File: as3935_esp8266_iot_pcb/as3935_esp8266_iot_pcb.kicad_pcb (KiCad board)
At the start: 2 copper layers, 50 x 100 mm, 44 parts, among them K1 RELAY_2RT, K2 RELAY_2RT, P1 CONN_01X02, P10 CONN_01X03, P2 CONN_01X02, P3 CONN_01X02, P5 CONN_01X07, P6 CONN_01X03, P7 CONN_01X05, P8 CONN_01X06, P9 CONN_01X01, Q1 Q_NPN_BCE, Q2 Q_NPN_BCE, SW1 SW_FLASH, SW2 SW_RESET, U1 PC817, U2 as3935, U3 ESP-12, U4 ESP-201, U5 AP1117D33

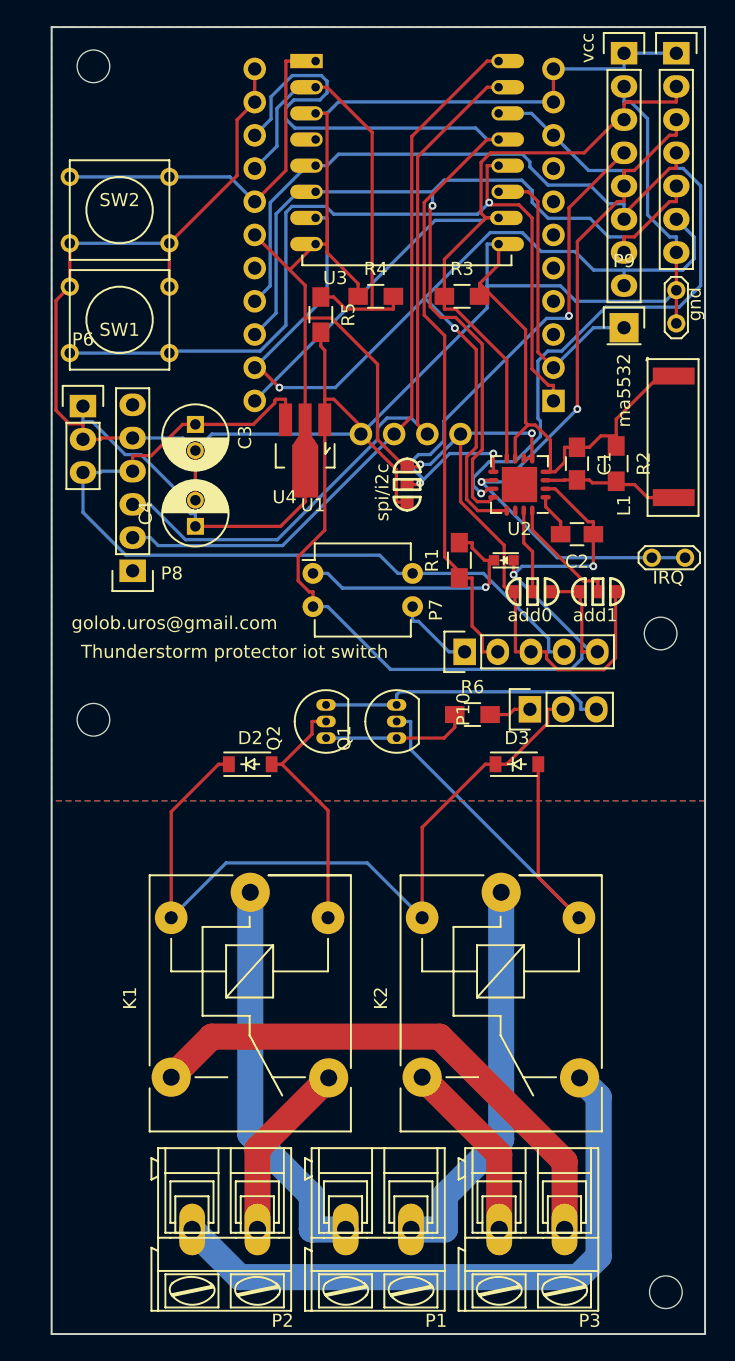
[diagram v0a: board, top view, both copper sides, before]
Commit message: small redesign
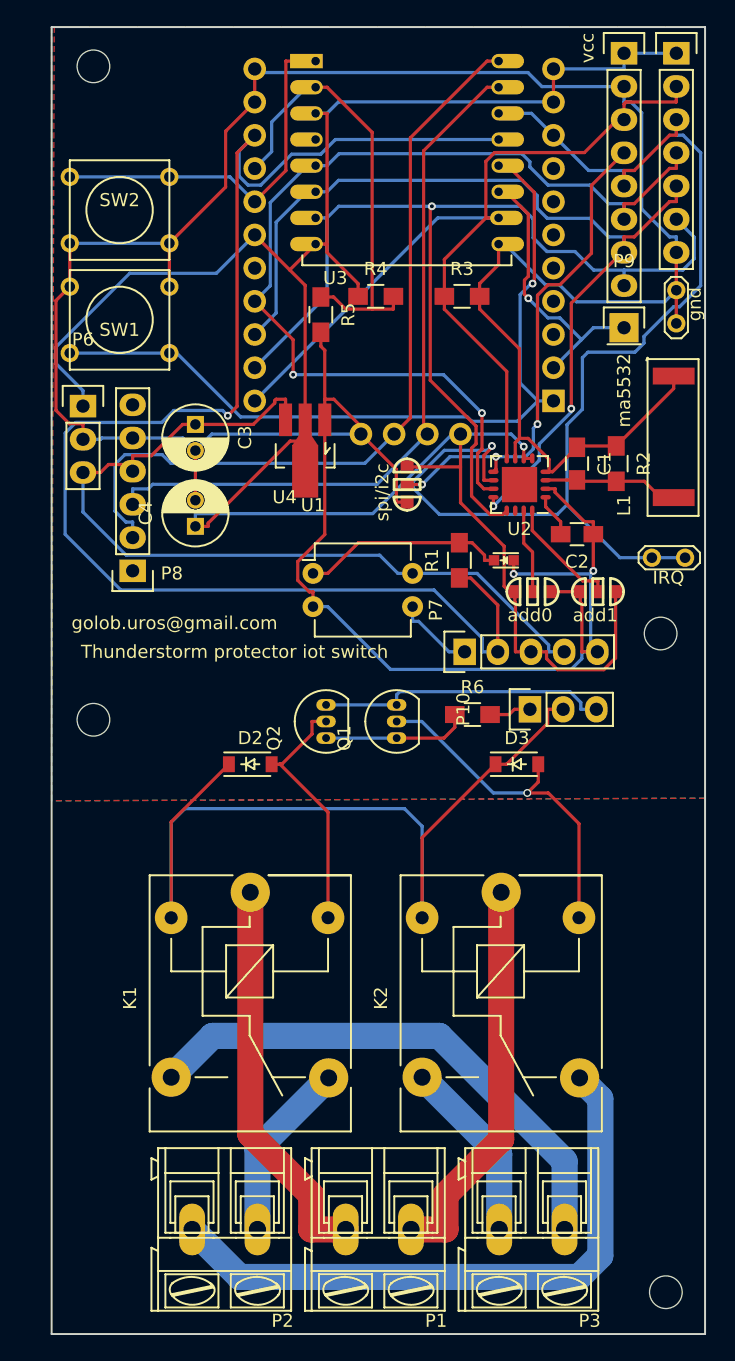
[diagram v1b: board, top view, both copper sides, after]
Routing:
- net /to_sw: track 76.8 -> 113.4 mm, vias 0 -> 1
- net /irq: track 67.5 -> 92.1 mm, vias 2 -> 1
- net +3V3: track 158.4 -> 173.8 mm, vias 2 -> 1
- net /clk: track 87.6 -> 76.5 mm, vias 1 -> 2
- net +5V: track 123.9 -> 134.7 mm
- net Net-(D3-Pad2): track 34.5 -> 26.9 mm, vias 0 -> 1
- net /tx: track 56.2 -> 61.7 mm
- net /flash: track 64.9 -> 60.4 mm
- net /si: track 42.5 -> 38.1 mm
- net GND: track 277.7 -> 281.6 mm
- net /miso: track 76.5 -> 72.7 mm, vias 1 -> 2
- net Net-(D1-Pad2): track 19.3 -> 15.6 mm, vias 1 -> 0
- net /rx: track 58.5 -> 55.0 mm
- net /mosi: track 80.9 -> 78.3 mm, vias 2 -> 1
- net Net-(P9-Pad1): track 23.2 -> 21.7 mm, vias 0 -> 1
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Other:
- net class ac: clearance 0.6 -> 0.65
